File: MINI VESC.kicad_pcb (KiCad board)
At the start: 4 copper layers, 65 x 18 mm, 151 parts, among them P1 CONN_1, P10 CONN_01X06, P11 CONN_01X06, P2 CONN_1, P3 CONN_1, P4 CONN_1, P5 CONN_1, P6 CONN_1, P9 CONN_01X06, Q1 NTMFS5C604NLT1G, Q2 NTMFS5C604NLT1G, Q3 NTMFS5C604NLT1G, Q4 NTMFS5C604NLT1G, Q5 NTMFS5C604NLT1G, Q6 NTMFS5C604NLT1G, U1 LM5113, U10 MCP1700, U2 LM5113, U3 LM5113, U4 AD8418, U5 AD8418, U6 AD8418, U7 STM32F40X_LQFP64, U8 LMR16006, U9 MCP1700, X1 ABM3B-8.000MHZ

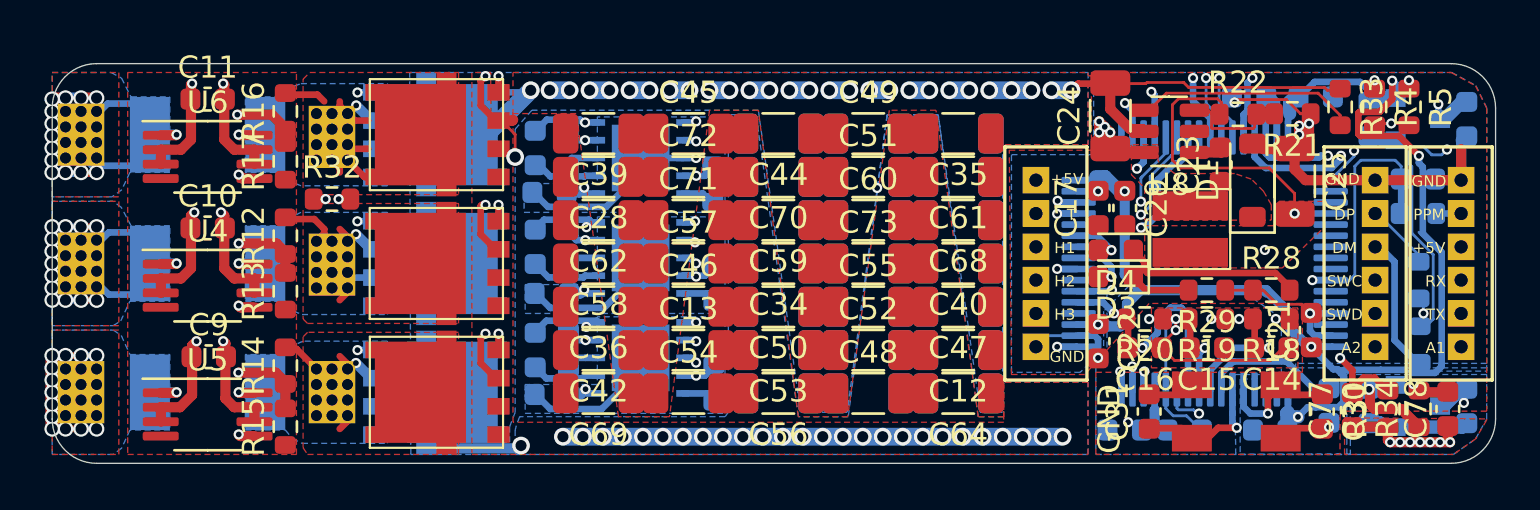
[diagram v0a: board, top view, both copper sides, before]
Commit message: More work
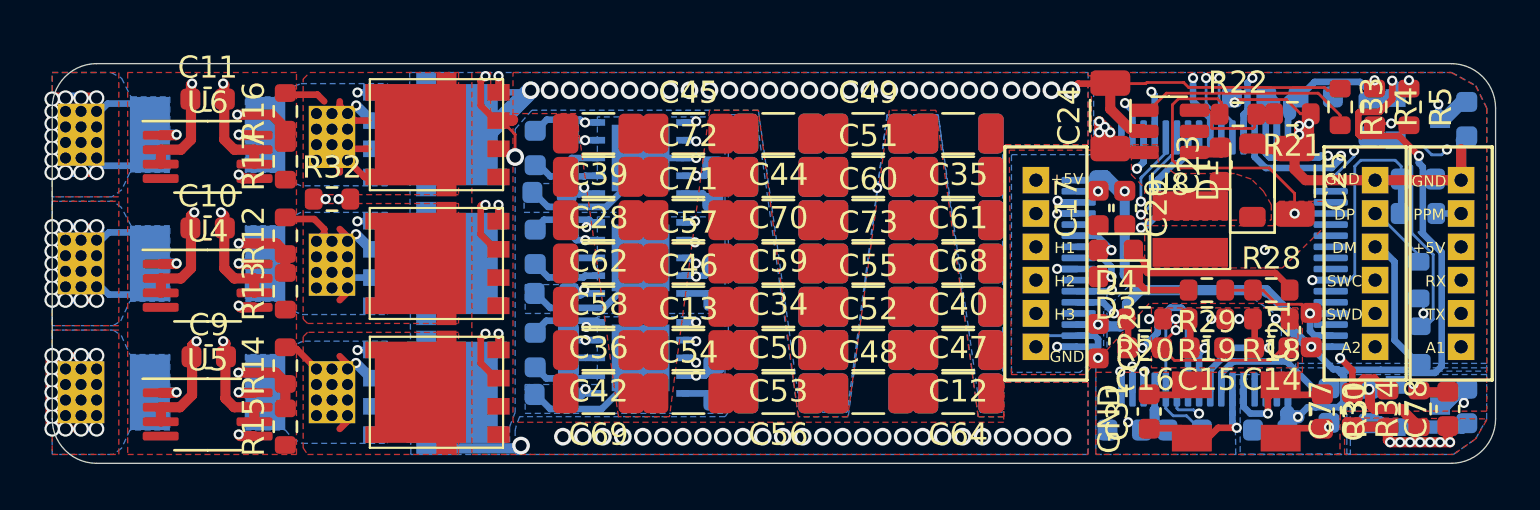
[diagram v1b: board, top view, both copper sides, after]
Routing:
- net VSS: track 321.1 -> 298.6 mm
- net VDD: track 105.7 -> 93.0 mm
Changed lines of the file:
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@@
   (segment (start 132.52 85.07) (end 130.85 83.4) (width 0.127) (layer "In1.Cu") (net 1))
   (segment (start 88.2825 83.295) (end 89.455 83.295) (width 0.3) (layer "B.Cu") (net 1))
-  (segment (start 92.2 83.2) (end 93.1 83.2) (width 0.8) (layer "B.Cu") (net 1))
-  (segment (start 90.4 83.2) (end 91.3 83.2) (width 0.8) (layer "B.Cu") (net 1))
-  (segment (start 97.6 83.2) (end 98.5 83.2) (width 0.8) (layer "B.Cu") (net 1))
   (segment (start 84.8425 99.3275) (end 88.985466 99.3275) (width 0.46) (layer "B.Cu") (net 1))
-  (segment (start 104.8 83.2) (end 105.7 83.2) (width 0.8) (layer "B.Cu") (net 1))
   (segment (start 86.0175 85.2) (end 87.55 85.2) (width 0.8) (layer "B.Cu") (net 1))
   (segment (start 89.455 83.295) (end 89.55 83.2) (width 0.3) (layer "B.Cu") (net 1))
-  (segment (start 108.4 83.2) (end 109.3 83.2) (width 0.8) (layer "B.Cu") (net 1))
-  (segment (start 94 83.2) (end 94.9 83.2) (width 0.8) (layer "B.Cu") (net 1))
   (segment (start 88.985466 99.3275) (end 89.113216 99.19975) (width 0.46) (layer "B.Cu") (net 1))
-  (segment (start 113 83.2) (end 113.9 83.2) (width 0.8) (layer "B.Cu") (net 1))
-  (segment (start 101.2 83.2) (end 102.1 83.2) (width 0.8) (layer "B.Cu") (net 1))
   (segment (start 87.55 85.2) (end 89.55 83.2) (width 0.8) (layer "B.Cu") (net 1))
-  (segment (start 99.4 83.2) (end 100.3 83.2) (width 0.8) (layer "B.Cu") (net 1))
-  (segment (start 95.8 83.2) (end 96.7 83.2) (width 0.8) (layer "B.Cu") (net 1))
   (segment (start 86.0175 85.2) (end 87.2 85.2) (width 0.8) (layer "B.Cu") (net 1))
-  (segment (start 110.2 83.2) (end 111.2 83.2) (width 0.8) (layer "B.Cu") (net 1))
   (segment (start 86.0175 96.8) (end 87.177002 96.8) (width 0.46) (layer "B.Cu") (net 1))
-  (segment (start 103 83.2) (end 103.9 83.2) (width 0.8) (layer "B.Cu") (net 1))
-  (segment (start 106.6 83.2) (end 107.5 83.2) (width 0.8) (layer "B.Cu") (net 1))
-  (segment (start 111.2 83.2) (end 112.1 83.2) (width 0.8) (layer "B.Cu") (net 1))
   (segment (start 81.746359 89.096639) (end 81.742998 89.1) (width 0.46) (layer "In1.Cu") (net 2))
   (segment (start 81.742998 89.1) (end 82.068267 89.1) (width 0.46) (layer "In2.Cu") (net 2))
@@
   (segment (start 90.427001 93.002001) (end 92.847999 93.002001) (width 0.3) (layer "B.Cu") (net 4))
   (segment (start 89.75 96.9) (end 89.775 96.9) (width 0.3) (layer "B.Cu") (net 4))
-  (segment (start 106.3 98.8) (end 107.2 98.8) (width 0.8) (layer "B.Cu") (net 4))
-  (segment (start 112.6 98.8) (end 113.5 98.8) (width 0.8) (layer "B.Cu") (net 4))
   (segment (start 92.946601 88.452001) (end 94.5 86.898602) (width 0.3) (layer "B.Cu") (net 4))
   (segment (start 92.747999 97.552001) (end 94.5 95.8) (width 0.3) (layer "B.Cu") (net 4))
@@
   (segment (start 118.14994 96.75056) (end 118.14994 97.5278) (width 0.127) (layer "B.Cu") (net 4))
   (segment (start 115.1 94.400758) (end 114.950442 94.2512) (width 0.3) (layer "B.Cu") (net 4))
-  (segment (start 102.7 98.8) (end 103.6 98.8) (width 0.8) (layer "B.Cu") (net 4))
   (segment (start 92.847999 93.002001) (end 94.5 91.35) (width 0.3) (layer "B.Cu") (net 4))
   (segment (start 94.5 91.35) (end 94.5 90.75) (width 0.3) (layer "B.Cu") (net 4))
-  (segment (start 109 98.8) (end 109.9 98.8) (width 0.8) (layer "B.Cu") (net 4))
   (segment (start 131.45 85.5) (end 131.7 85.25) (width 0.46) (layer "B.Cu") (net 4))
   (segment (start 118.48214 97.86) (end 119.085 97.86) (width 0.127) (layer "B.Cu") (net 4))
-  (segment (start 109.9 98.8) (end 110.8 98.8) (width 0.8) (layer "B.Cu") (net 4))
-  (segment (start 97.3 98.8) (end 98.2 98.8) (width 0.8) (layer "B.Cu") (net 4))
   (segment (start 127.95 85.45) (end 128.5 85.45) (width 0.6) (layer "B.Cu") (net 4))
-  (segment (start 110.8 98.8) (end 111.7 98.8) (width 0.8) (layer "B.Cu") (net 4))
-  (segment (start 111.7 98.8) (end 112.6 98.8) (width 0.8) (layer "B.Cu") (net 4))
-  (segment (start 103.6 98.8) (end 104.5 98.8) (width 0.8) (layer "B.Cu") (net 4))
   (segment (start 115.1 95.25) (end 115.1 94.400758) (width 0.3) (layer "B.Cu") (net 4))
-  (segment (start 98.2 98.8) (end 99.1 98.8) (width 0.8) (layer "B.Cu") (net 4))
   (segment (start 94.5 95.8) (end 94.5 95.25) (width 0.3) (layer "B.Cu") (net 4))
   (segment (start 127.3 98.167242) (end 127.767242 98.167242) (width 0.6) (layer "B.Cu") (net 4))
   (segment (start 131.5 98.367242) (end 128.5 98.367242) (width 0.6) (layer "B.Cu") (net 4))
-  (segment (start 100 98.8) (end 100.9 98.8) (width 0.8) (layer "B.Cu") (net 4))
   (segment (start 89.65 87.8) (end 89.675 87.8) (width 0.3) (layer "B.Cu") (net 4))
   (segment (start 89.675 87.8) (end 90.327001 88.452001) (width 0.3) (layer "B.Cu") (net 4))
   (segment (start 114.14944 94.2512) (end 112.7988 94.2512) (width 0.127) (layer "B.Cu") (net 4))
-  (segment (start 91 98.8) (end 91.9 98.8) (width 0.8) (layer "B.Cu") (net 4))
-  (segment (start 92.8 98.8) (end 93.7 98.8) (width 0.8) (layer "B.Cu") (net 4))
   (segment (start 96.4 90.75) (end 96.742998 90.75) (width 0.3) (layer "B.Cu") (net 4))
   (segment (start 127.767242 98.167242) (end 127.967242 98.367242) (width 0.6) (layer "B.Cu") (net 4))
-  (segment (start 96.4 98.8) (end 97.3 98.8) (width 0.8) (layer "B.Cu") (net 4))
   (segment (start 114.950442 94.2512) (end 114.14944 94.2512) (width 0.3) (layer "B.Cu") (net 4))
   (segment (start 119.725 98.5) (end 119.75 98.5) (width 0.127) (layer "B.Cu") (net 4))
   (segment (start 96.4 86.25) (end 96.995124 86.25) (width 0.3) (layer "B.Cu") (net 4))
-  (segment (start 101.8 98.8) (end 102.7 98.8) (width 0.8) (layer "B.Cu") (net 4))
-  (segment (start 105.4 98.8) (end 106.3 98.8) (width 0.8) (layer "B.Cu") (net 4))
   (segment (start 128.7 99.05) (end 128.25 99.05) (width 0.127) (layer "B.Cu") (net 4))
   (segment (start 131.45 87.25) (end 131.45 85.5) (width 0.46) (layer "B.Cu") (net 4))
@@
   (segment (start 89.775 96.9) (end 90.427001 97.552001) (width 0.3) (layer "B.Cu") (net 4))
   (segment (start 121.15 83.5) (end 121.15 83.643987) (width 0.127) (layer "B.Cu") (net 4))
-  (segment (start 94.6 98.8) (end 95.5 98.8) (width 0.8) (layer "B.Cu") (net 4))
   (segment (start 124.852098 94.2512) (end 125.65056 94.2512) (width 0.3) (layer "B.Cu") (net 4))
-  (segment (start 99.1 98.8) (end 100 98.8) (width 0.8) (layer "B.Cu") (net 4))
   (segment (start 118.14994 96.75056) (end 118.14994 93.950059) (width 0.127) (layer "B.Cu") (net 4))
   (segment (start 129.6 99.05) (end 129.15 99.05) (width 0.127) (layer "B.Cu") (net 4))
   (segment (start 127.3 85.25) (end 127.75 85.25) (width 0.6) (layer "B.Cu") (net 4))
-  (segment (start 93.7 98.8) (end 94.6 98.8) (width 0.8) (layer "B.Cu") (net 4))
   (segment (start 131.45 87.25) (end 130.3 87.25) (width 0.46) (layer "B.Cu") (net 4))
   (segment (start 118.14994 93.950059) (end 118.6 93.499999) (width 0.127) (layer "B.Cu") (net 4))
@@
   (segment (start 118.14994 97.5278) (end 118.48214 97.86) (width 0.127) (layer "B.Cu") (net 4))
   (segment (start 115.154009 84.604009) (end 115.4 84.85) (width 0.127) (layer "B.Cu") (net 4))
-  (segment (start 107.2 98.8) (end 108.1 98.8) (width 0.8) (layer "B.Cu") (net 4))
-  (segment (start 95.5 98.8) (end 96.4 98.8) (width 0.8) (layer "B.Cu") (net 4))
   (segment (start 112.7988 94.2512) (end 112.3 94.75) (width 0.127) (layer "B.Cu") (net 4))
   (segment (start 131.7 98.167242) (end 131.7 98.3) (width 0.127) (layer "B.Cu") (net 4))
   (segment (start 96.995124 86.25) (end 96.997562 86.247562) (width 0.3) (layer "B.Cu") (net 4))
-  (segment (start 100.9 98.8) (end 101.8 98.8) (width 0.8) (layer "B.Cu") (net 4))
   (segment (start 124.643318 93.25) (end 124.643318 94.04242) (width 0.3) (layer "B.Cu") (net 4))
   (segment (start 130.3 87.25) (end 130.25 87.2) (width 0.46) (layer "B.Cu") (net 4))
-  (segment (start 108.1 98.8) (end 109 98.8) (width 0.8) (layer "B.Cu") (net 4))
   (segment (start 96.4 95.25) (end 96.779887 95.25) (width 0.3) (layer "B.Cu") (net 4))
   (segment (start 115.15 84.604009) (end 115.154009 84.604009) (width 0.127) (layer "B.Cu") (net 4))
-  (segment (start 91.9 98.8) (end 92.8 98.8) (width 0.8) (layer "B.Cu") (net 4))
-  (segment (start 104.5 98.8) (end 105.4 98.8) (width 0.8) (layer "B.Cu") (net 4))
   (segment (start 96.4 86.25) (end 94.5 86.25) (width 0.3) (layer "B.Cu") (net 4))
   (segment (start 127.967242 98.367242) (end 128.5 98.367242) (width 0.6) (layer "B.Cu") (net 4))
